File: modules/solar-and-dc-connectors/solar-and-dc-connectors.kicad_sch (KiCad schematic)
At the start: 3 parts, among them J1 S2B-PH-K-SLFSN, J2 54-00127

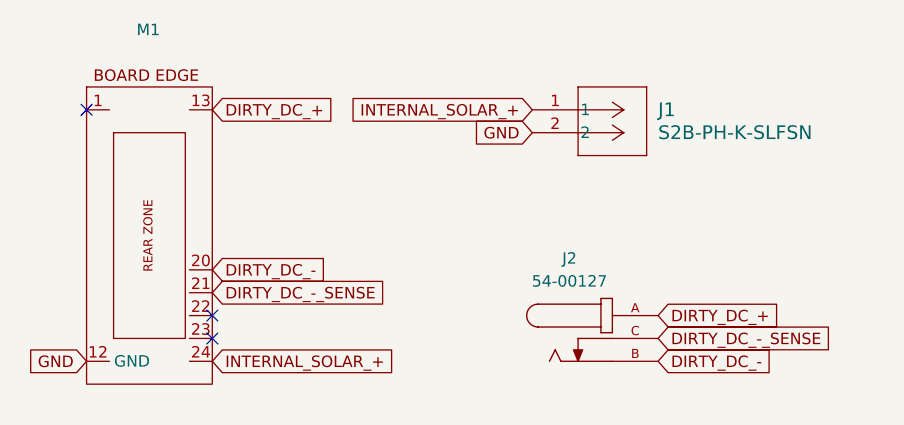
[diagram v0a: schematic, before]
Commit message: Updating all modules
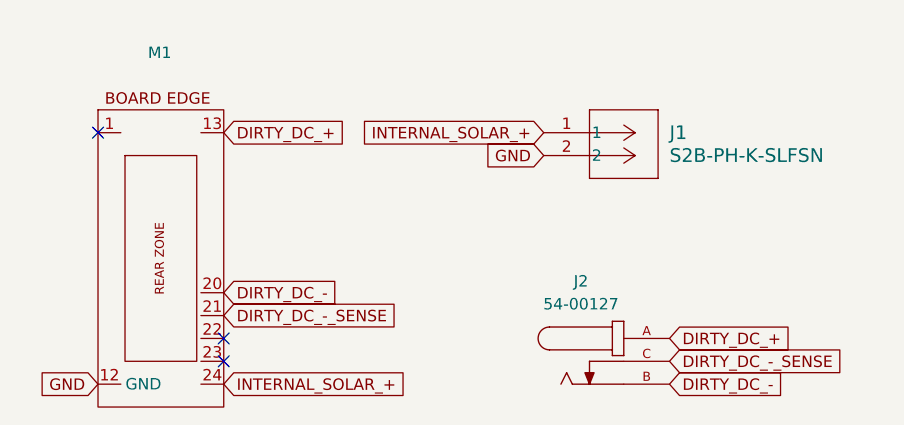
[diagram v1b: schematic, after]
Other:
- moved on the sheet: J1, J2, M1
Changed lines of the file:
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@@
 	(paper "A4")
 	(no_connect
-		(at 53.34 46.99)
+		(at 54.61 49.53)
 	)
 	(no_connect
-		(at 67.31 69.85)
+		(at 68.58 72.39)
 	)
 	(no_connect
-		(at 67.31 72.39)
+		(at 68.58 74.93)
 	)
 	(global_label "DIRTY_DC_-_SENSE"
 		(shape input)
-		(at 67.31 67.31 0)
-		(fields_autoplaced yes)
-		(effects
-			(font
-				(size 1.27 1.27)
-			)
-			(justify left)
-		)
-		(property "Intersheetrefs" "${INTERSHEET_REFS}"
-			(at 88.5589 67.31 0)
+		(at 68.58 69.85 0)
+		(fields_autoplaced yes)
+		(effects
+			(font
+				(size 1.27 1.27)
+			)
+			(justify left)
+		)
+		(property "Intersheetrefs" "${INTERSHEET_REFS}"
+			(at 89.8289 69.85 0)
 			(effects
 				(font
@@
 	(global_label "DIRTY_DC_-"
 		(shape input)
-		(at 116.84 74.93 0)
-		(fields_autoplaced yes)
-		(effects
-			(font
-				(size 1.27 1.27)
-			)
-			(justify left)
-		)
-		(property "Intersheetrefs" "${INTERSHEET_REFS}"
-			(at 131.0738 74.93 0)
+		(at 118.11 77.47 0)
+		(fields_autoplaced yes)
+		(effects
+			(font
+				(size 1.27 1.27)
+			)
+			(justify left)
+		)
+		(property "Intersheetrefs" "${INTERSHEET_REFS}"
+			(at 132.3438 77.47 0)
 			(effects
 				(font
@@
 	(global_label "INTERNAL_SOLAR_+"
 		(shape input)
-		(at 67.31 74.93 0)
-		(fields_autoplaced yes)
-		(effects
-			(font
-				(size 1.27 1.27)
-			)
-			(justify left)
-		)
-		(property "Intersheetrefs" "${INTERSHEET_REFS}"
-			(at 88.4986 74.93 0)
+		(at 68.58 77.47 0)
+		(fields_autoplaced yes)
+		(effects
+			(font
+				(size 1.27 1.27)
+			)
+			(justify left)
+		)
+		(property "Intersheetrefs" "${INTERSHEET_REFS}"
+			(at 89.7686 77.47 0)
 			(effects
 				(font
@@
 	(global_label "GND"
 		(shape input)
-		(at 53.34 74.93 180)
+		(at 54.61 77.47 180)
 		(fields_autoplaced yes)
 		(effects
@@
 		)
 		(property "Intersheetrefs" "${INTERSHEET_REFS}"
-			(at 46.4843 74.93 0)
+			(at 47.7543 77.47 0)
 			(effects
 				(font
@@
 	(global_label "DIRTY_DC_-"
 		(shape input)
-		(at 67.31 64.77 0)
-		(fields_autoplaced yes)
-		(effects
-			(font
-				(size 1.27 1.27)
-			)
-			(justify left)
-		)
-		(property "Intersheetrefs" "${INTERSHEET_REFS}"
-			(at 81.5438 64.77 0)
+		(at 68.58 67.31 0)
+		(fields_autoplaced yes)
+		(effects
+			(font
+				(size 1.27 1.27)
+			)
+			(justify left)
+		)
+		(property "Intersheetrefs" "${INTERSHEET_REFS}"
+			(at 82.8138 67.31 0)
 			(effects
 				(font
@@
 	(global_label "INTERNAL_SOLAR_+"
 		(shape input)
-		(at 102.87 46.99 180)
+		(at 104.14 49.53 180)
 		(fields_autoplaced yes)
 		(effects
@@
 		)
 		(property "Intersheetrefs" "${INTERSHEET_REFS}"
-			(at 81.6814 46.99 0)
+			(at 82.9514 49.53 0)
 			(effects
 				(font
@@
 	(global_label "DIRTY_DC_+"
 		(shape input)
-		(at 67.31 46.99 0)
-		(fields_autoplaced yes)
-		(effects
-			(font
-				(size 1.27 1.27)
-			)
-			(justify left)
-		)
-		(property "Intersheetrefs" "${INTERSHEET_REFS}"
-			(at 81.5438 46.99 0)
+		(at 68.58 49.53 0)
+		(fields_autoplaced yes)
+		(effects
+			(font
+				(size 1.27 1.27)
+			)
+			(justify left)
+		)
+		(property "Intersheetrefs" "${INTERSHEET_REFS}"
+			(at 82.8138 49.53 0)
 			(effects
 				(font
@@
 	(global_label "DIRTY_DC_+"
 		(shape input)
-		(at 116.84 69.85 0)
-		(fields_autoplaced yes)
-		(effects
-			(font
-				(size 1.27 1.27)
-			)
-			(justify left)
-		)
-		(property "Intersheetrefs" "${INTERSHEET_REFS}"
-			(at 131.0738 69.85 0)
+		(at 118.11 72.39 0)
+		(fields_autoplaced yes)
+		(effects
+			(font
+				(size 1.27 1.27)
+			)
+			(justify left)
+		)
+		(property "Intersheetrefs" "${INTERSHEET_REFS}"
+			(at 132.3438 72.39 0)
 			(effects
 				(font
@@
 	(global_label "GND"
 		(shape input)
-		(at 102.87 49.53 180)
+		(at 104.14 52.07 180)
 		(fields_autoplaced yes)
 		(effects
@@
 		)
 		(property "Intersheetrefs" "${INTERSHEET_REFS}"
-			(at 96.0143 49.53 0)
+			(at 97.2843 52.07 0)
 			(effects
 				(font
@@
 	(global_label "DIRTY_DC_-_SENSE"
 		(shape input)
-		(at 116.84 72.39 0)
-		(fields_autoplaced yes)
-		(effects
-			(font
-				(size 1.27 1.27)
-			)
-			(justify left)
-		)
-		(property "Intersheetrefs" "${INTERSHEET_REFS}"
-			(at 138.0889 72.39 0)
+		(at 118.11 74.93 0)
+		(fields_autoplaced yes)
+		(effects
+			(font
+				(size 1.27 1.27)
+			)
+			(justify left)
+		)
+		(property "Intersheetrefs" "${INTERSHEET_REFS}"
+			(at 139.3589 74.93 0)
 			(effects
 				(font
@@
 	(symbol
 		(lib_id "MegaCastle:MegaCastle2x12-Module-I12.5x25.7-M80181F-EDGE")
-		(at 59.69 60.96 0)
+		(at 60.96 63.5 0)
 		(unit 1)
 		(exclude_from_sim no)
@@
 		(fields_autoplaced yes)
 		(property "Reference" "M1"
-			(at 60.1938 38.1 0)
+			(at 61.4638 40.64 0)
 			(effects
 				(font
@@
 		)
 		(property "Value" "~"
-			(at 60.1938 40.64 0)
+			(at 61.4638 43.18 0)
 			(effects
 				(font
@@
 		)
 		(property "Footprint" "MegaCastle:MegaCastle2x12-Module-I20.0x25.7-M80181F-SPAREPAD"
-			(at 59.69 82.55 0)
+			(at 60.96 85.09 0)
 			(effects
 				(font
@@
 		)
 		(property "Datasheet" ""
-			(at 59.69 55.88 0)
+			(at 60.96 58.42 0)
 			(effects
 				(font
@@
 		)
 		(property "Description" "Generated using footprint-gen .. 12.5 25.4 8 M80181F"
-			(at 59.69 60.96 0)
+			(at 60.96 63.5 0)
 			(effects
 				(font
@@
 	(symbol
 		(lib_id "2025-03-05_08-59-15:S2B-PH-K-SLFSN")
-		(at 102.87 46.99 0)
+		(at 104.14 49.53 0)
 		(unit 1)
 		(exclude_from_sim no)
@@
 		(fields_autoplaced yes)
 		(property "Reference" "J1"
-			(at 116.84 46.9899 0)
+			(at 118.11 49.5299 0)
 			(effects
 				(font
@@
 		)
 		(property "Value" "S2B-PH-K-SLFSN"
-			(at 116.84 49.5299 0)
+			(at 118.11 52.0699 0)
 			(effects
 				(font
@@
 		)
 		(property "Footprint" "MegaCastle:CONN_S2B-PH-K-S_JST"
-			(at 102.87 46.99 0)
+			(at 104.14 49.53 0)
 			(effects
 				(font
@@
 		)
 		(property "Datasheet" "https://eu.mouser.com/datasheet/2/564/ePH-3433490.pdf"
-			(at 102.87 46.99 0)
+			(at 104.14 49.53 0)
 			(effects
 				(font
@@
 		)
 		(property "Description" ""
-			(at 102.87 46.99 0)
+			(at 104.14 49.53 0)
 			(effects
 				(font
@@
 		)
 		(property "Mouser" "https://eu.mouser.com/ProductDetail/JST-Commercial/S2B-PH-K-SLFSN?qs=cdbOS8ANM9A5Ie4gXeMjTA%3D%3D"
-			(at 102.87 46.99 0)
+			(at 104.14 49.53 0)
 			(effects
 				(font
@@
 		)
 		(property "Mouser PN" "306-S2BPHKSLFSNPP"
-			(at 102.87 46.99 0)
+			(at 104.14 49.53 0)
 			(effects
 				(font
@@
 		)
 		(property "Mfr. PN" " S2B-PH-K-S(LF)(SN) "
-			(at 102.87 46.99 0)
+			(at 104.14 49.53 0)
 			(effects
 				(font
@@
 	(symbol
 		(lib_id "54-00127:54-00127")
-		(at 111.76 72.39 0)
+		(at 113.03 74.93 0)
 		(unit 1)
 		(exclude_from_sim no)
@@
 		(fields_autoplaced yes)
 		(property "Reference" "J2"
-			(at 107.0003 63.5 0)
+			(at 108.2703 66.04 0)
 			(effects
 				(font
@@
 		)
 		(property "Value" "54-00127"
-			(at 107.0003 66.04 0)
+			(at 108.2703 68.58 0)
 			(effects
 				(font
@@
 		)
 		(property "Footprint" "MegaCastle:TENSILITY_54-00127"
-			(at 111.76 72.39 0)
+			(at 113.03 74.93 0)
 			(effects
 				(font
@@
 		)
 		(property "Datasheet" "https://tensility.s3.us-west-2.amazonaws.com/uploads/pdffiles/54-00127.pdf"
-			(at 111.76 72.39 0)
+			(at 113.03 74.93 0)
 			(effects
 				(font
@@
 		)
 		(property "Description" ""
-			(at 111.76 72.39 0)
+			(at 113.03 74.93 0)
 			(effects
 				(font
@@
 		)
 		(property "PARTREV" "A"
-			(at 111.76 72.39 0)
+			(at 113.03 74.93 0)
 			(effects
 				(font
@@
 		)
 		(property "STANDARD" "Manufacturer Recommendations"
-			(at 111.76 72.39 0)
+			(at 113.03 74.93 0)
 			(effects
 				(font
@@
 		)
 		(property "SNAPEDA_PN" "54-00127"
-			(at 111.76 72.39 0)
+			(at 113.03 74.93 0)
 			(effects
 				(font
@@
 		)
 		(property "MAXIMUM_PACKAGE_HEIGHT" "7.3mm"
-			(at 111.76 72.39 0)
+			(at 113.03 74.93 0)
 			(effects
 				(font
@@
 		)
 		(property "MANUFACTURER" "TENSILITY"
-			(at 111.76 72.39 0)
+			(at 113.03 74.93 0)
 			(effects
 				(font
@@
 		)
 		(property "Digikey" "https://www.digikey.com/en/products/detail/tensility-international-corp/54-00127/9685436"
-			(at 111.76 72.39 0)
-			(effects
-				(font
+			(at 113.03 74.93 0)
+			(effects
+				(font
